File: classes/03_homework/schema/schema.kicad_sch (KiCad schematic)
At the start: 11 parts

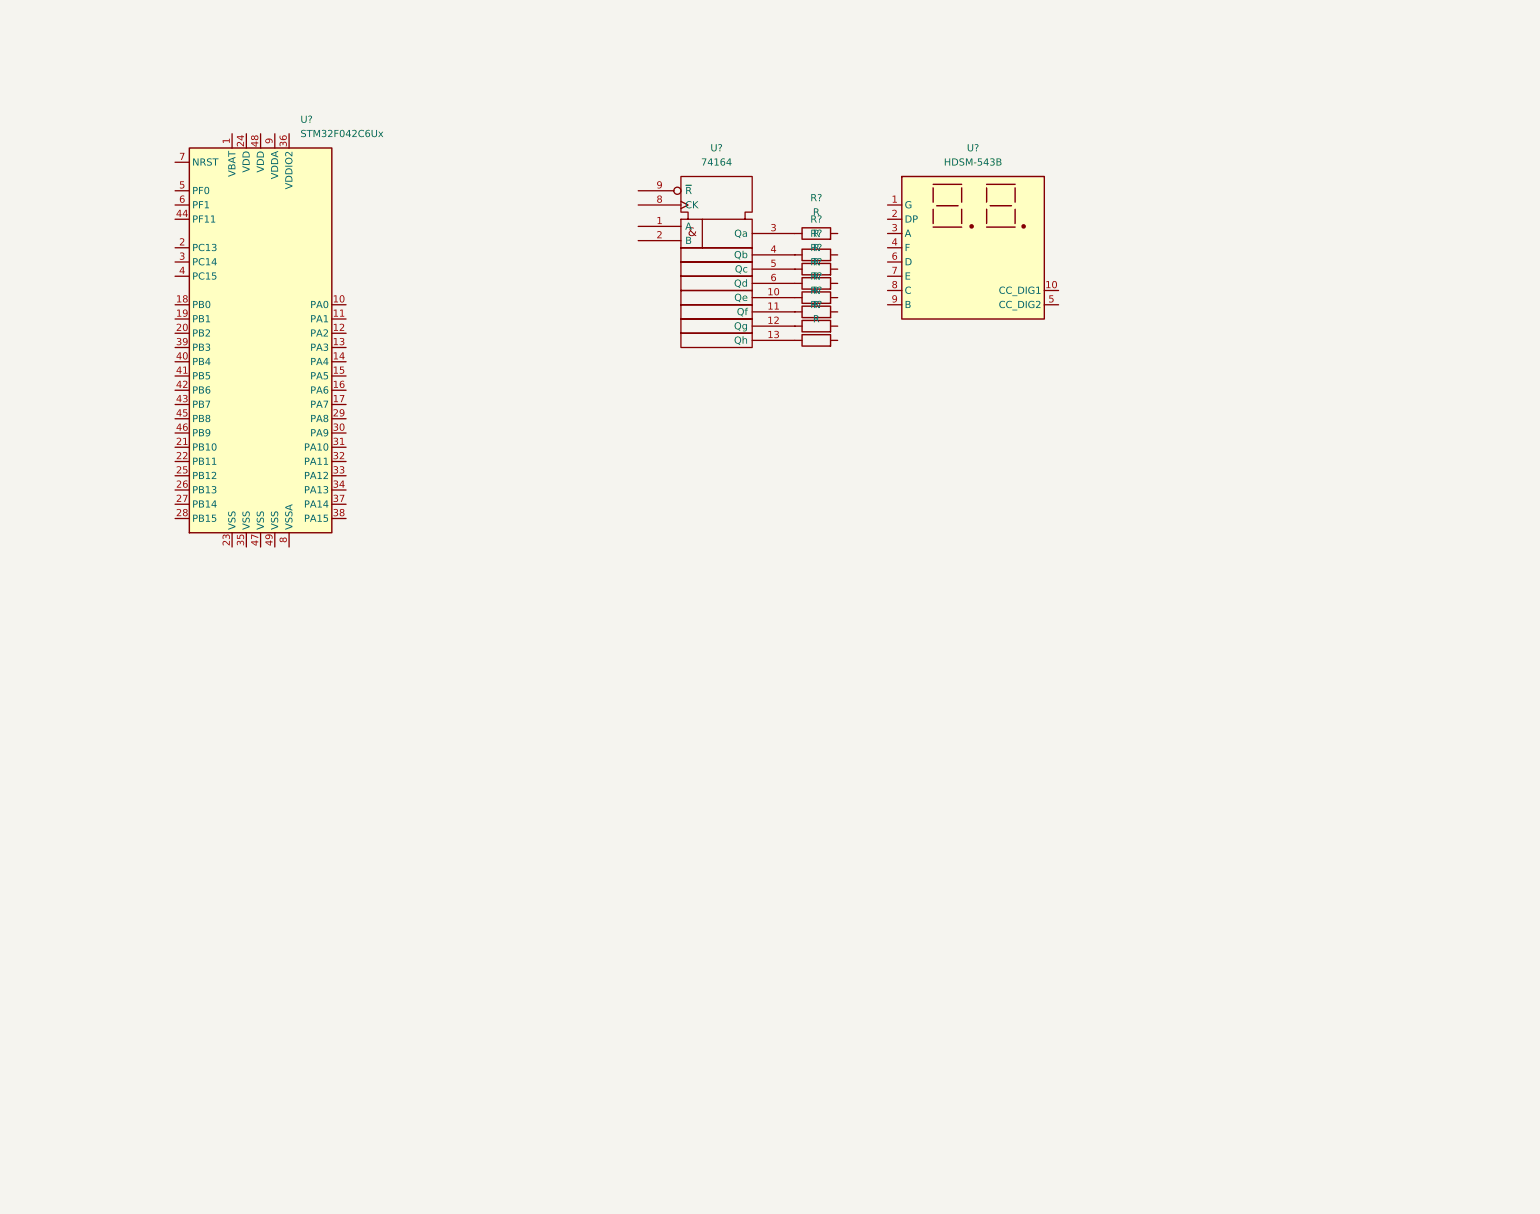
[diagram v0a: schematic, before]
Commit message: Upload task schema
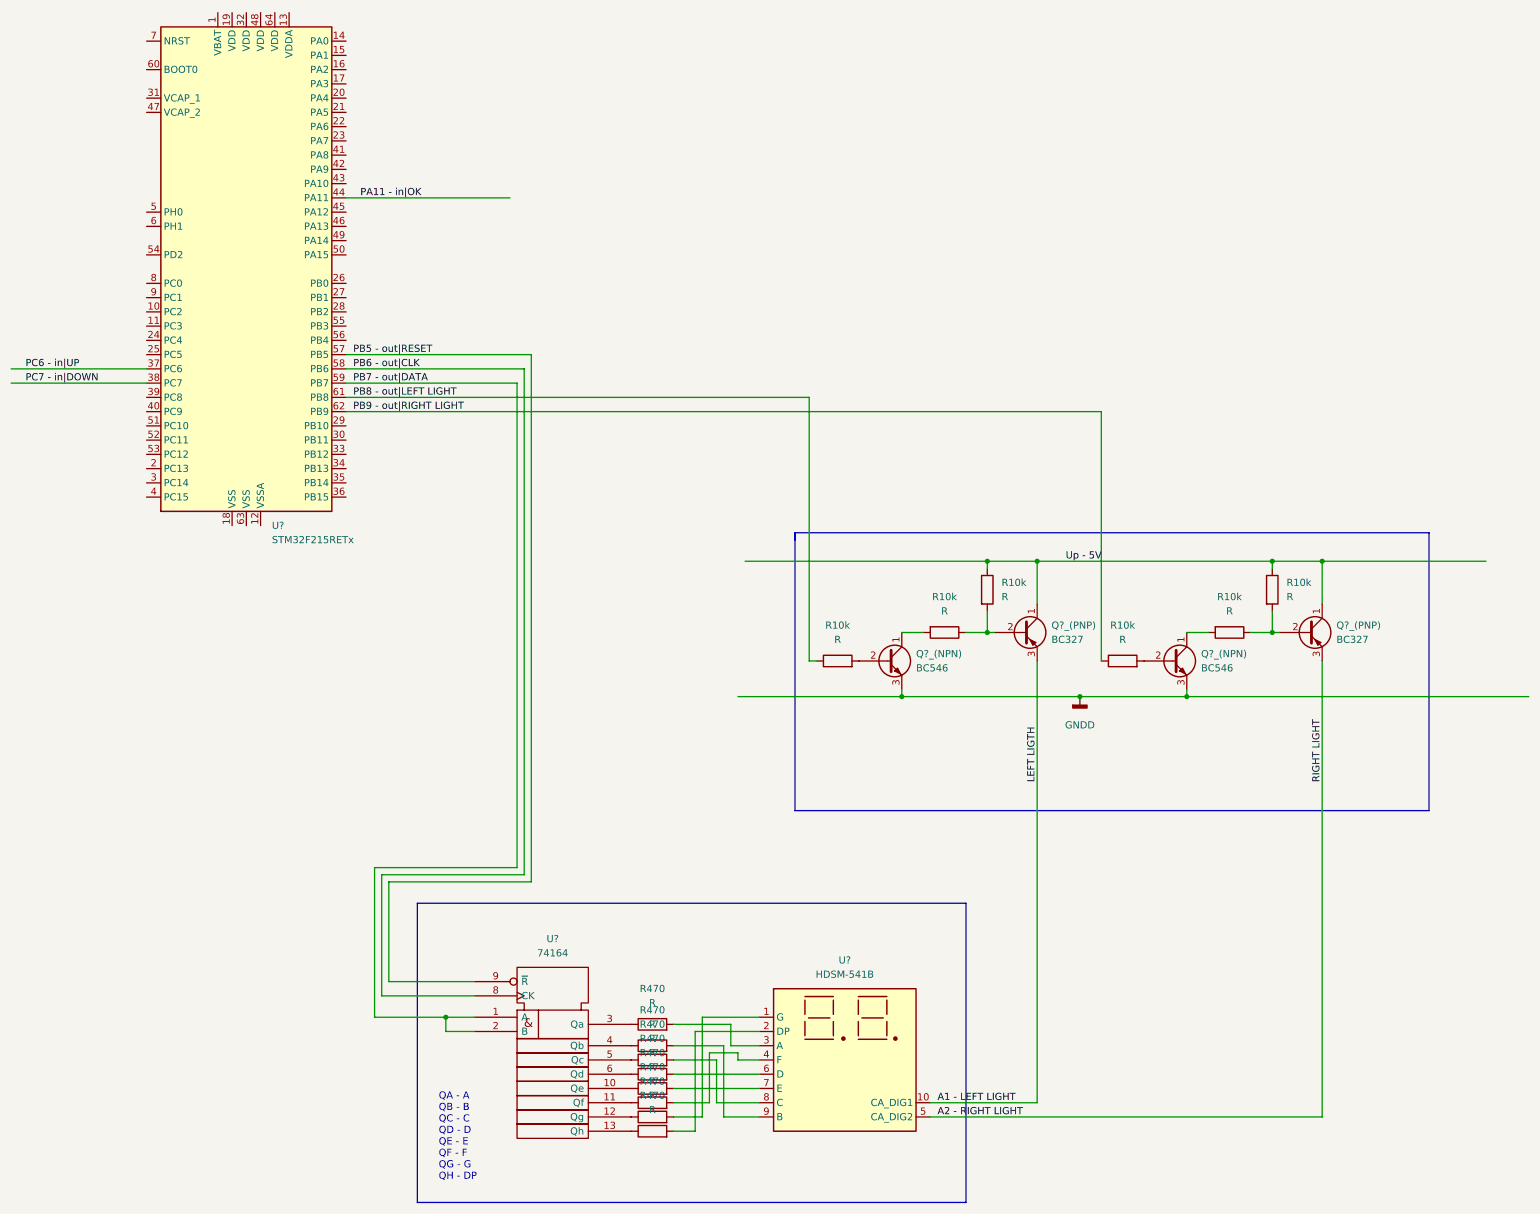
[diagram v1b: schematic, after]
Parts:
- removed R? (x8): R, symbol Device:R
- removed U?: 74164, symbol 74xx_IEEE:74164
- removed U?: HDSM-543B, Display:HDSM-541B_HDSM-543B, symbol Display_Character:HDSM-543B
- removed U?: STM32F042C6Ux, Package_DFN_QFN:QFN-48-1EP_7x7mm_P0.5mm_EP5.6x5.6mm, symbol MCU_ST_STM32F0:STM32F042C6Ux
- added Q?_(NPN) (x2): BC546, Package_TO_SOT_THT:TO-92_Inline, symbol Transistor_BJT:BC546
- added Q?_(PNP) (x2): BC327, Package_TO_SOT_THT:TO-92_Inline, symbol Transistor_BJT:BC327
- added R10k (x6), R470 (x8): R, symbol Device:R
- added U?: STM32F215RETx, Package_QFP:LQFP-64_10x10mm_P0.5mm, symbol MCU_ST_STM32F2:STM32F215RETx
- added U?: 74164, symbol 74xx_IEEE:74164
- added U?: HDSM-541B, Display:HDSM-441B_HDSM-443B, symbol Display_Character:HDSM-541B
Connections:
- net Vdd: now also U?.14 (Vdd)
- net Vss: now also U?.7 (Vss)
- new net: R470.1, U?.5 (Qc)
- new net: R470.2, U?.8 (C)
- new net: Q?_(PNP).2 (B), R10k.1, R10k.2 (x2)
- new net: Q?_(NPN).1 (C), R10k.2 (x2)
- new net: R470.1, U?.3 (Qa)
- new net: R470.2, U?.3 (A)
- new net: Q?_(NPN).2 (B), R10k.2 (x2)
- new net: R470.1, U?.6 (Qd)
- new net: R470.2, U?.6 (D)
- new net: R470.1, U?.10 (Qe)
- new net: R470.2, U?.7 (E)
- new net: R470.1, U?.12 (Qg)
- new net: R470.2, U?.1 (G)
- new net: R470.1, U?.4 (Qb)
- new net: R470.2, U?.9 (B)
- new net: R470.1, U?.11 (Qf)
- new net: R470.1, U?.13 (Qh)
- new net: R470.2, U?.2 (DP)
- new net: R470.2, U?.4 (F)
- new net A1 - LEFT LIGHT: Q?_(PNP).3 (E), U?.10 (CA_DIG1)
- new net A2 - RIGHT LIGHT: Q?_(PNP).3 (E), U?.5 (CA_DIG2)
- new net GNDD: Q?_(NPN).3 (E), Q?_(NPN).3 (E)
- new net PA11 - in|OK: U?.44 (PA11)
- new net PB5 - out|RESET: U?.57 (PB5), U?.9 (~{R})
- new net PB6 - out|CLK: U?.58 (PB6), U?.8 (CK)
- new net PB7 - out|DATA: U?.1 (A), U?.2 (B), U?.59 (PB7)
- new net PB8 - out|LEFT LIGHT: R10k.1, U?.61 (PB8)
- new net PB9 - out|RIGHT LIGHT: R10k.1, U?.62 (PB9)
- new net PC6 - in|UP: U?.37 (PC6)
- new net PC7 - in|DOWN: U?.38 (PC7)
- new net Up - 5V: Q?_(PNP).1 (C), Q?_(PNP).1 (C), R10k.1, R10k.1
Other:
- note added: "QA - A QB - B QC - C QD - D QE - E QF - F QG - G QH - DP"
